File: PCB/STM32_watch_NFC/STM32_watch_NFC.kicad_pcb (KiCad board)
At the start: 4 copper layers, 37 x 37 mm, 126 parts, among them J1 Conn_01x06_Socket, J2 USB_C_Receptacle_PowerOnly_6P, Q1 BC817, Q2 AO3400A, SW1 SW_DPST_x2, SW2 SW_DPST_x2, SW3 SW_DPST_x2, U1 BH1750FVI-TR, U2 74AHCT1G125, U3 STM32L031G6Ux, U4 LP5912-3.3DRV, U5 MCP73831-3-OT, U6 MT3608, Y1 32.768kHz

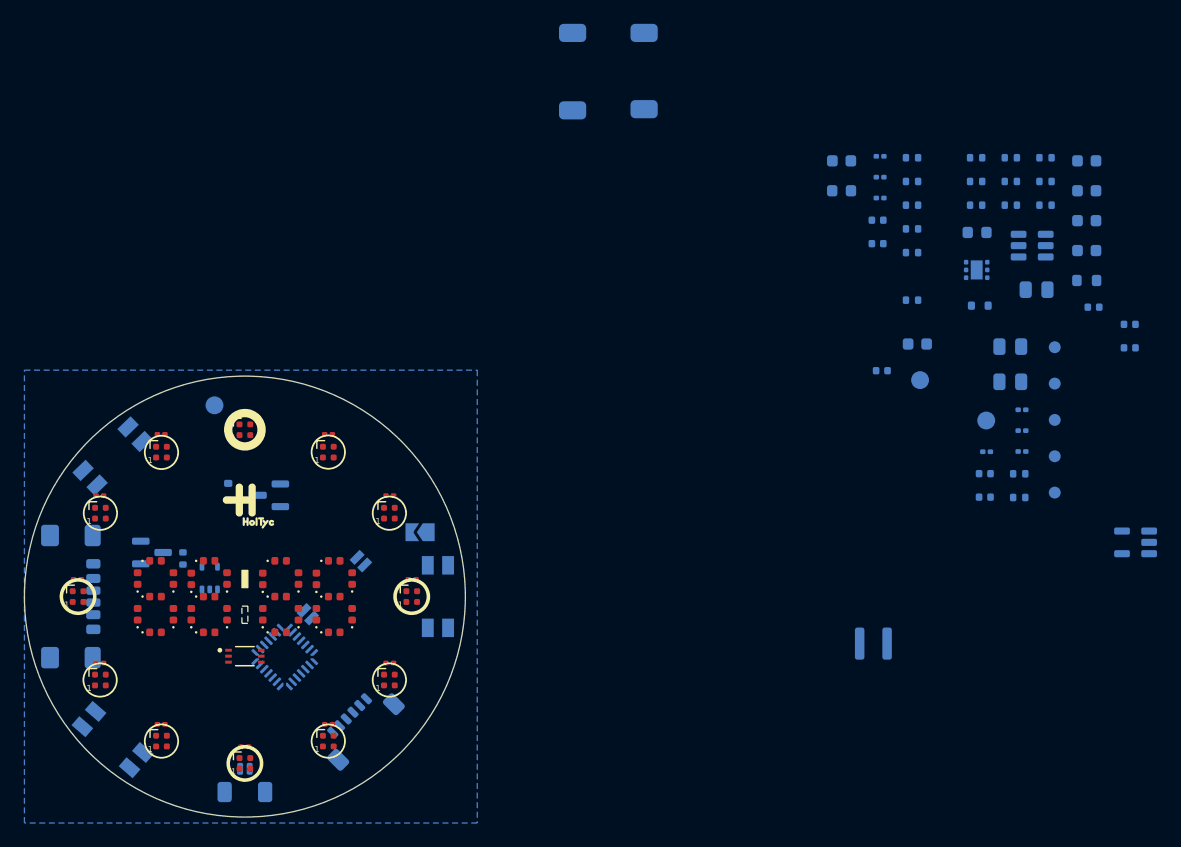
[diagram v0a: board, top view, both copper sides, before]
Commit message: Component placement
I placed every component in logical way
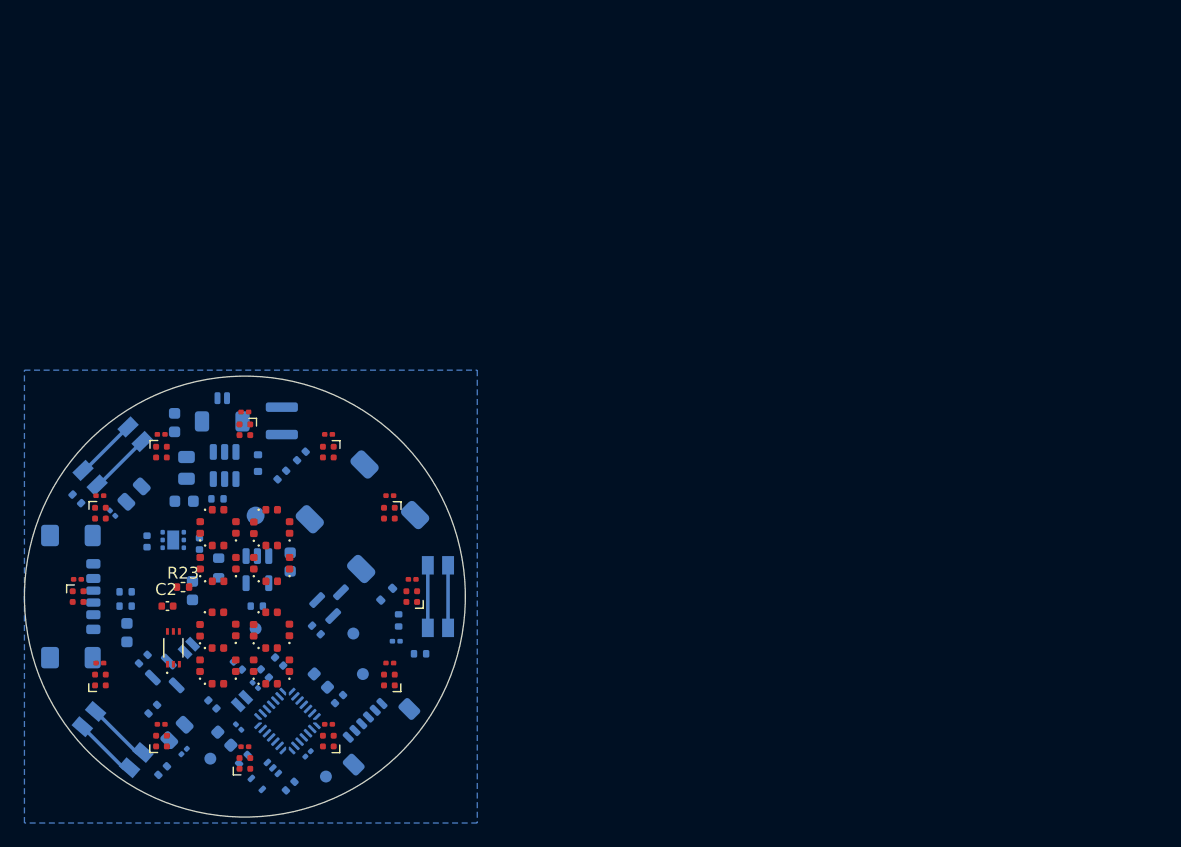
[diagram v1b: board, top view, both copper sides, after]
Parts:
- removed the C25 at (210.7, 92.8)
- removed D44: LED, LED_SMD:LED_0603_1608Metric
- removed G***: LOGO, LOGO
- removed GND, GND1: GND, TestPoint:TestPoint_Pad_D1.5mm
- removed JP1: SolderJumper_2_Open, Jumper:SolderJumper-2_P1.3mm_Open_TrianglePad1.0x1.5mm
- removed R1, R12, R2: 510, Resistor_SMD:R_0402_1005Metric
- added R23: 2.2K, Resistor_SMD:R_0402_1005Metric, F.Cu at (143.3, 104.2)
- C2: moved to F.Cu
- moved R17 83.5 mm to (140.8, 114.4), turned to 45 degrees
- moved C12 83.3 mm to (145.8, 114.0), turned to 135 degrees
- moved R15 83.3 mm to (138.5, 105.8), turned to 0 degrees
- moved C29 83.3 mm to (144.1, 104.5), turned to -90 degrees
- moved R16 81.9 mm to (138.5, 104.6)
- moved C28 81.8 mm to (140.3, 100.4), turned to -90 degrees
- moved R20 80.6 mm to (140.0, 110.2), turned to 45 degrees
- moved C13 79.4 mm to (147.9, 110.8), turned to 135 degrees
- moved C31 79.3 mm to (143.4, 97.0), turned to 0 degrees
- moved R4 79.1 mm to (134.4, 96.8), turned to -45 degrees
- moved R6 78.8 mm to (141.6, 119.6), turned to 45 degrees
- moved C32 77.9 mm to (142.6, 90.4), turned to -90 degrees
- moved DINL 77.5 mm to (145.6, 118.6)
- moved C3 76.8 mm to (143.4, 118.0), turned to -135 degrees
- moved C1 76.8 mm to (137.4, 98.0), turned to 135 degrees
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- renumbered +BAT1 to BAT, Buzzer_d1 to Buz, DINLED1 to DINL, DINSTM1 to DINS, SCL_L1 to SCL, SDA_L1 to SDA
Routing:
- net +3.3V: track 0.00 -> 15.9 mm
- net Net-(SW1A-A): track 0.00 -> 5.39 mm
- net Net-(SW3A-A): track 0.00 -> 5.29 mm
- net Net-(SW2A-A): track 0.00 -> 5.25 mm

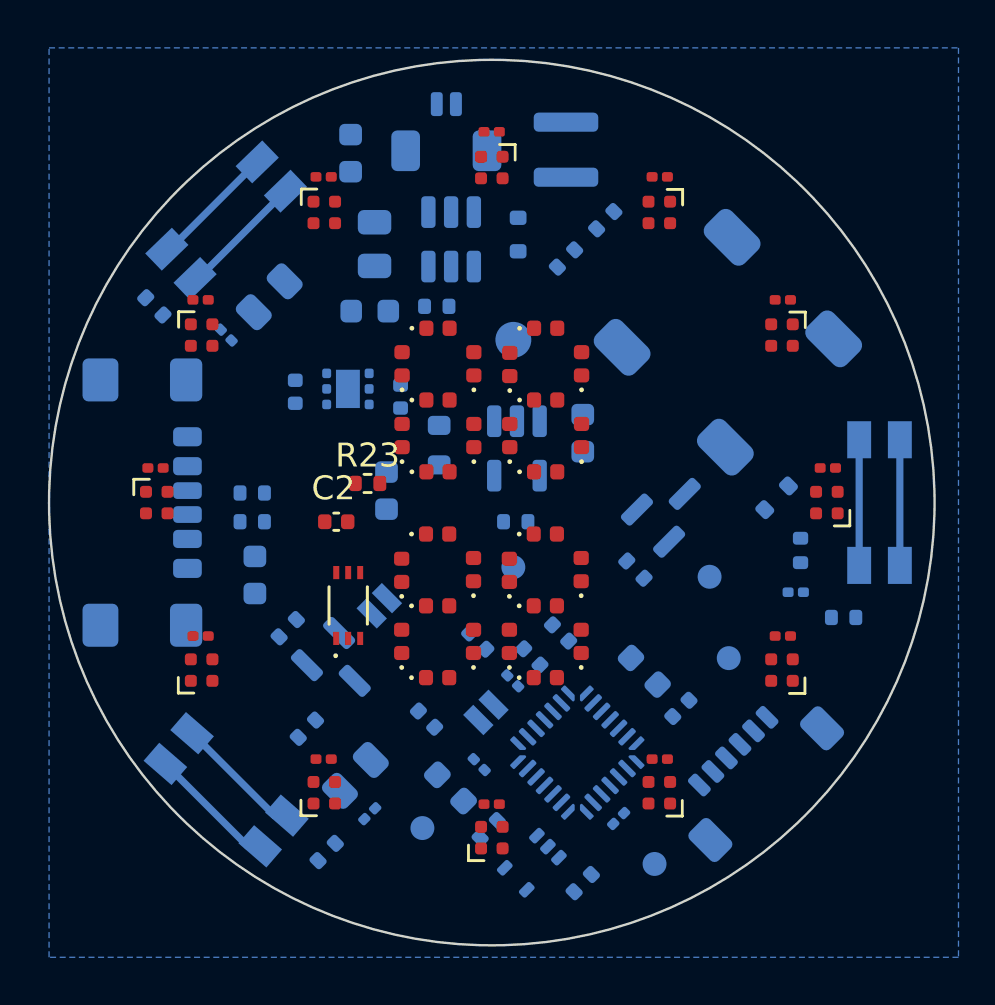
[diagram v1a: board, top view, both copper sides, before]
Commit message: Routing #1
Starting routing
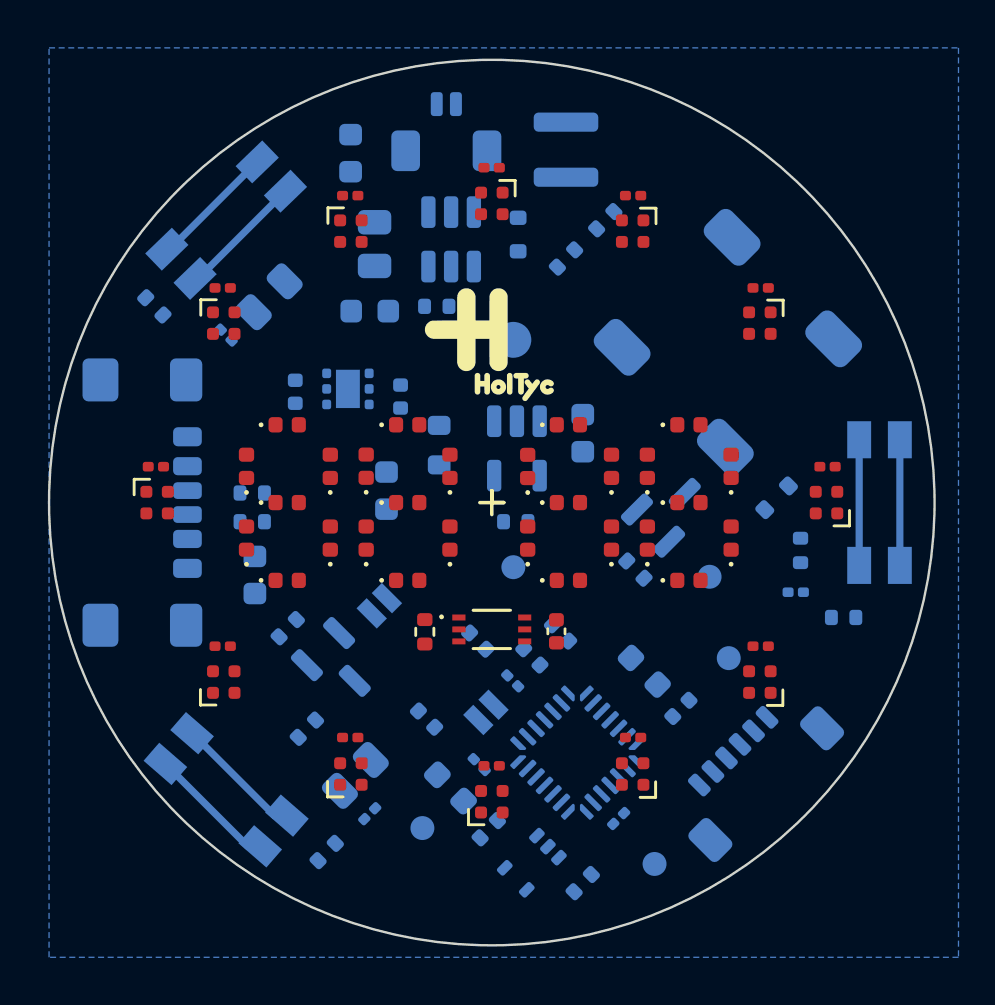
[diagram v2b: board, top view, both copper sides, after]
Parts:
- added G***: LOGO, LOGO, F.Cu at (148.8, 98.5)
- moved C2 10.3 mm to (151.2, 110.4), turned to -90 degrees
- moved D17 7.79 mm to (138.2, 106.5)
- moved D18 7.79 mm to (138.2, 103.5)
- moved D16 7.76 mm to (139.9, 108.2)
- moved D19 7.62 mm to (139.9, 105.0)
- moved D35 7.61 mm to (158.5, 103.5)
- moved D36 7.61 mm to (158.5, 106.5)
- moved D34 7.54 mm to (156.7, 101.8)
- moved D13 7.48 mm to (139.9, 101.8)
- moved D40 7.39 mm to (156.7, 105.0)
- moved D14 7.37 mm to (141.8, 103.5)
- moved D15 7.37 mm to (141.8, 106.5)
- moved D24 7.37 mm to (143.2, 106.5)
- moved D25 7.35 mm to (143.2, 103.5)
- moved D23 7.33 mm to (145.0, 108.2)
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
